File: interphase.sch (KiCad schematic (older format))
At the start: 1 part

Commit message: schematic preversion and layout preversion
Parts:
- added BT1: Battery_Cell, symbol Battery_Cell
- added C1: 4,7µF, Capacitors_SMD:C_0805_HandSoldering, symbol C
- added C2: 10µF, Capacitors_SMD:C_0805_HandSoldering, symbol C
- added D1, D10, D11, D12, D13, D14, D15, D16, D17, D18, D19, D2, D20, D21, D22, D23, D24, D25, D26, D27, D28, D29, D3, D30, D31, D32, D33, D34, D35, D4, D5, D6, D7, D8, D9: D, Diodes_SMD:D_MiniMELF, symbol D
- added L1: 4,7µH, symbol L
- added R1: 536K, symbol R
- added R2: 309K, symbol R
- added R3: 100K, symbol R
- added SW1, SW10, SW11, SW12, SW13, SW14, SW15, SW16, SW17, SW18, SW19, SW2, SW20, SW21, SW22, SW23, SW24, SW25, SW26, SW27, SW28, SW29, SW3, SW30, SW31, SW32, SW33, SW34, SW35, SW36, SW4, SW5, SW6, SW7, SW8, SW9: MOM-SPST, Misc:CHERRY-MX, symbol MOM-SPST
- added U2: MCP1640, TO_SOT_Packages_SMD:SOT-23-6, symbol MCP1640
- gave numbers to parts that had none: 1
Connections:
- net GND: now reaches U1.1 (GND)
- net GND: now also U1.11 (GND), BT1.2 (-), C1.2, C2.2, R2.2, R3.2, U2.2 (GND)
- net +3V3: now reaches U1.12 (VCC)
- net +3V3: now also C2.1, R1.1, U2.5 (VOUT)
- net at U1.15 (P01): now also BT1.1 (+), C1.1, L1.1, SW1.1, U2.6 (VIN)
- net at U1.23 (P09): now also D31.1 (K)
- net at U1.24 (P10): now also D26.1 (K)
- net at U1.25 (P11): now also D21.1 (K)
- net at U1.26 (P12): now also D16.1 (K)
- net at U1.27 (P13): now also D11.1 (K)
- net at U1.28 (P14): now also D6.1 (K)
- net at U1.29 (P15): now also D1.1 (K), D2.1 (K), D3.1 (K), D4.1 (K), D5.1 (K)
- net at U1.30 (P16): now also SW11.1, SW16.1, SW21.1, SW26.1, SW31.1, SW36.1, SW6.1
- net at U1.33 (P17): now also SW10.1, SW15.1, SW20.1, SW25.1, SW30.1, SW35.1, SW5.1
- net at U1.34 (P18): now also SW14.1, SW19.1, SW24.1, SW29.1, SW34.1, SW4.1, SW9.1
- net at U1.35 (P19): now also SW13.1, SW18.1, SW23.1, SW28.1, SW3.1, SW33.1, SW8.1
- net at U1.36 (P20): now also SW12.1, SW17.1, SW2.1, SW22.1, SW27.1, SW32.1, SW7.1
- new net: L1.2, U2.1 (SW)
- new net: R3.1, SW1.2, U2.3 (EN)
- new net: R1.2, R2.1, U2.4 (VFB)
- new net: D31.2 (A), SW32.2
- new net: D26.2 (A), SW27.2
- new net: D21.2 (A), SW22.2
- new net: D16.2 (A), SW17.2
- new net: D11.2 (A), SW12.2
- new net: D6.2 (A), SW7.2
- new net: D1.2 (A), SW2.2
- new net: D32.2 (A), SW33.2
- new net: D27.2 (A), SW28.2
- new net: D22.2 (A), SW23.2
- new net: D17.2 (A), SW18.2
- new net: D12.2 (A), SW13.2
- new net: D7.2 (A), SW8.2
- new net: D2.2 (A), SW3.2
- new net: D33.2 (A), SW34.2
- new net: D28.2 (A), SW29.2
- new net: D23.2 (A), SW24.2
- new net: D18.2 (A), SW19.2
- new net: D13.2 (A), SW14.2
- new net: D8.2 (A), SW9.2
- new net: D3.2 (A), SW4.2
- new net: D34.2 (A), SW35.2
- new net: D29.2 (A), SW30.2
- new net: D24.2 (A), SW25.2
- new net: D19.2 (A), SW20.2
- new net: D14.2 (A), SW15.2
- new net: D9.2 (A), SW10.2
- new net: D4.2 (A), SW5.2
- new net: D35.2 (A), SW36.2
- new net: D30.2 (A), SW31.2
- new net: D25.2 (A), SW26.2
- new net: D20.2 (A), SW21.2
- new net: D15.2 (A), SW16.2
- new net: D10.2 (A), SW11.2
- new net: D5.2 (A), SW6.2
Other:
- moved on the sheet: U1

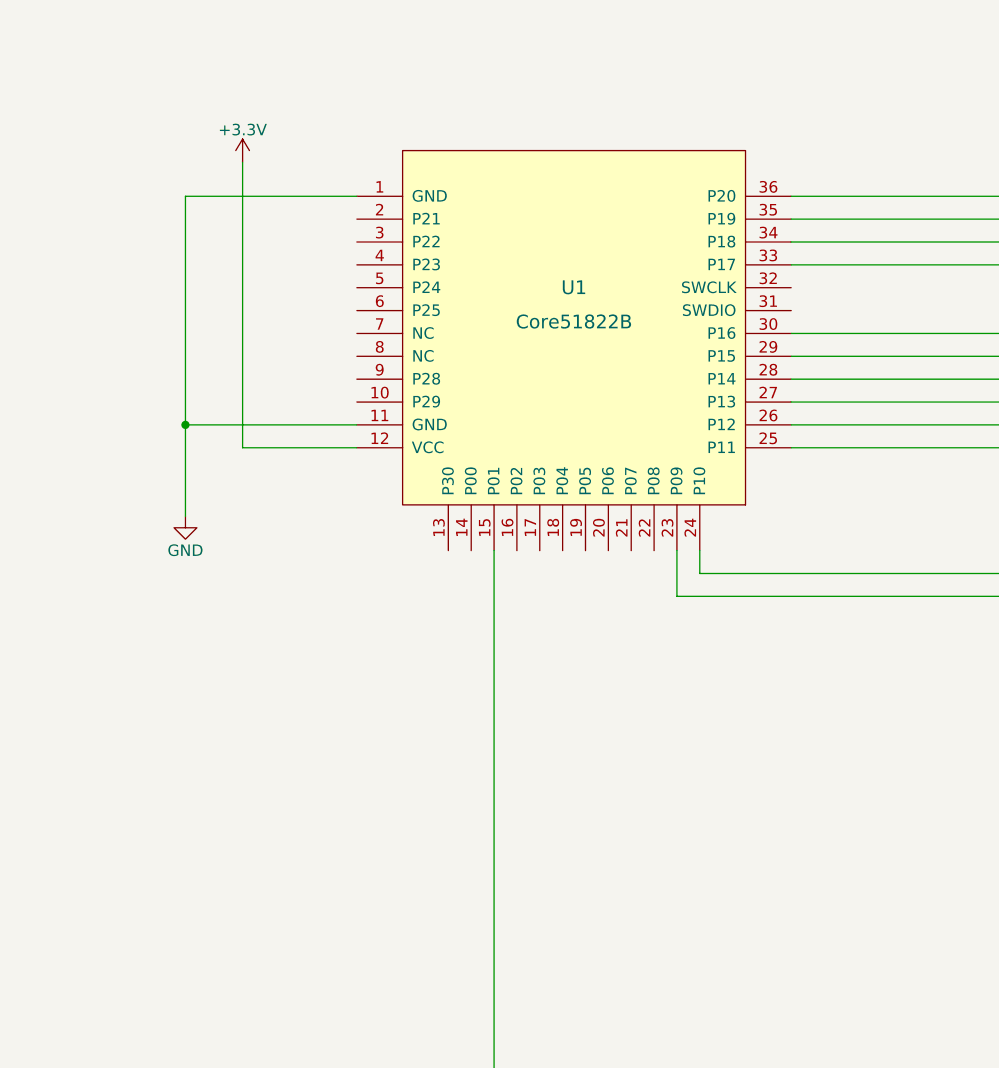
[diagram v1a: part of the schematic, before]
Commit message: some work
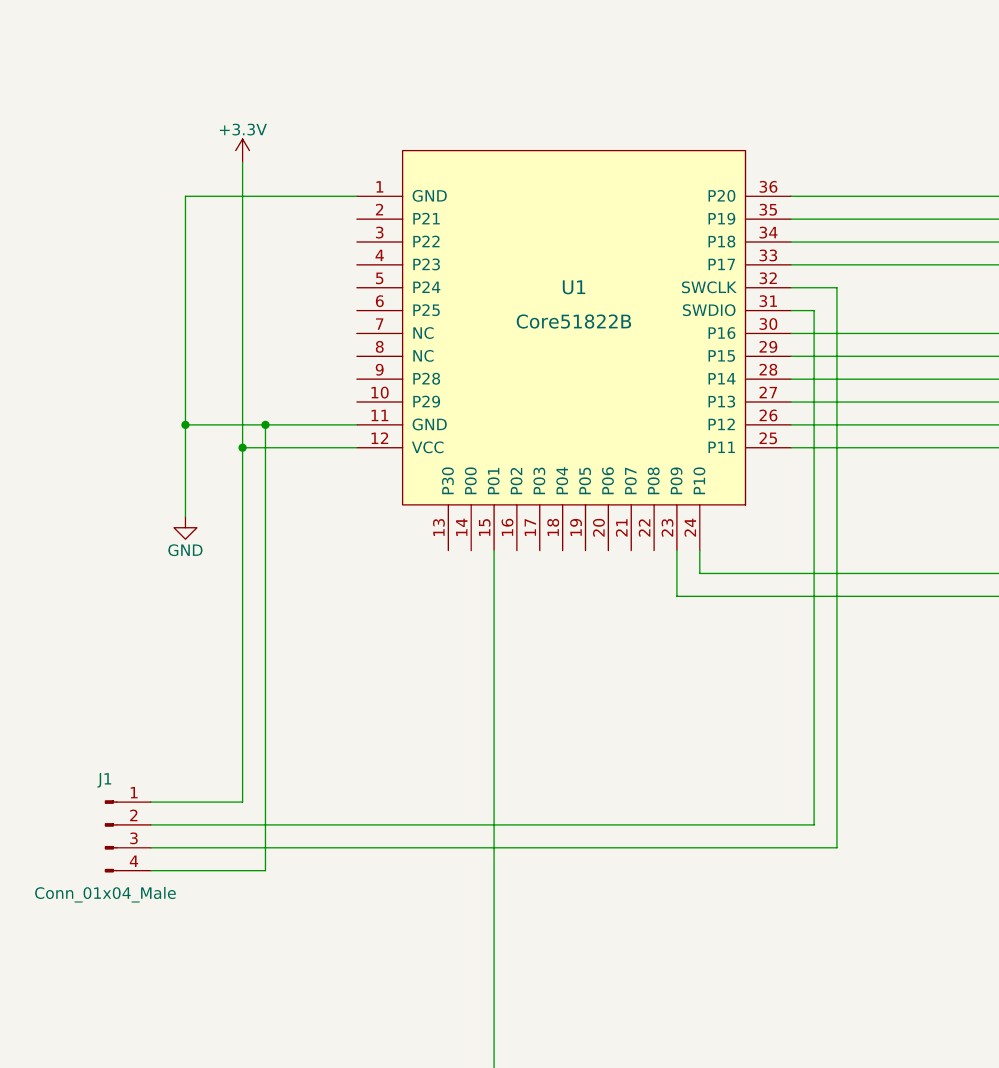
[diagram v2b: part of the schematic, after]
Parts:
- added J1: Conn_01x04_Male, symbol Conn_01x04_Male
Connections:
- net +3V3: now also J1.1 (Pin_1)
- net GND: now also J1.4 (Pin_4)
- net at U1.31 (SWDIO): now also J1.2 (Pin_2)
- net at U1.32 (SWCLK): now also J1.3 (Pin_3)
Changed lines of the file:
@@
 $EndComp
 $Comp
-L +3.3V #PWR01
+L +3.3V #PWR5
 U 1 1 59BBF369
 P 34400 -7050
-F 0 "#PWR01" H 34400 -7200 50  0001 C CNN
+F 0 "#PWR5" H 34400 -7200 50  0001 C CNN
 F 1 "+3.3V" H 34400 -6910 50  0000 C CNN
 F 2 "" H 34400 -7050 50  0001 C CNN
@@
 $EndComp
 $Comp
-L GND #PWR02
+L GND #PWR3
 U 1 1 59BBF383
 P 3150 7100
-F 0 "#PWR02" H 3150 6850 50  0001 C CNN
+F 0 "#PWR3" H 3150 6850 50  0001 C CNN
 F 1 "GND" H 3150 6950 50  0000 C CNN
 F 2 "" H 3150 7100 50  0001 C CNN
@@
 $EndComp
 $Comp
-L +3.3V #PWR03
+L +3.3V #PWR4
 U 1 1 59C15857
 P 5000 5950
-F 0 "#PWR03" H 5000 5800 50  0001 C CNN
+F 0 "#PWR4" H 5000 5800 50  0001 C CNN
 F 1 "+3.3V" H 5000 6090 50  0000 C CNN
 F 2 "" H 5000 5950 50  0001 C CNN
@@
 Connection ~ 2700 6350
 $Comp
-L +3.3V #PWR04
+L +3.3V #PWR2
 U 1 1 59C23ED5
 P 1600 650
-F 0 "#PWR04" H 1600 500 50  0001 C CNN
+F 0 "#PWR2" H 1600 500 50  0001 C CNN
 F 1 "+3.3V" H 1600 790 50  0000 C CNN
 F 2 "" H 1600 650 50  0001 C CNN
@@
 $EndComp
 $Comp
-L GND #PWR05
+L GND #PWR1
 U 1 1 59C23F89
 P 1350 2200
-F 0 "#PWR05" H 1350 1950 50  0001 C CNN
+F 0 "#PWR1" H 1350 1950 50  0001 C CNN
 F 1 "GND" H 1350 2050 50  0000 C CNN
 F 2 "" H 1350 2200 50  0001 C CNN
@@
 	2100 1900 1600 1900
 Wire Wire Line
-	1600 1900 1600 650
+	1600 650  1600 3450
+$Comp
+L Conn_01x04_Male J1
+U 1 1 59C3A25B
+P 1000 3550
+F 0 "J1" H 1000 3750 50  0000 C CNN
+F 1 "Conn_01x04_Male" H 1000 3250 50  0000 C CNN
+F 2 "" H 1000 3550 50  0001 C CNN
+F 3 "" H 1000 3550 50  0001 C CNN
+	1    1000 3550
+	1    0    0    -1
+$EndComp
+Wire Wire Line
+	1600 3450 1200 3450
+Connection ~ 1600 1900
+Wire Wire Line
+	1200 3550 4100 3550
+Wire Wire Line
+	4100 3550 4100 1300
+Wire Wire Line
+	4100 1300 4000 1300
+Wire Wire Line
+	1200 3650 4200 3650
+Wire Wire Line
+	4200 3650 4200 1200
+Wire Wire Line
+	4200 1200 4000 1200
+Wire Wire Line
+	1200 3750 1700 3750
+Wire Wire Line
+	1700 3750 1700 1800
+Connection ~ 1700 1800
 $EndSCHEMATC
